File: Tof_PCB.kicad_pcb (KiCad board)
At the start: 4 copper layers, 115 x 65 mm, 275 parts, among them J1 Screw_Terminal_01x02, J2 Screw_Terminal_01x02, J3 Screw_Terminal_01x02, J4 Conn_02x03_Odd_Even, J5 Conn_01x04, J6 Conn_01x04, J7 Screw_Terminal_01x02, M1 mounting_holes_laser, M2 mounting_holes_laser, M3 mounting_holes_laser, M4 mounting_holes_laser, SW1 SW_Push, U1 ATmega328PB-MU, U10 NC7WZ00K8X, U11 UMCC_50Ohm, U12 UMCC_50Ohm, U13 NC7WZ00K8X, U14 NCP81074BDR2G, U15 LMH6559MF, U16 SiPM-MicroRB, U17 UMCC_50Ohm, U18 ts5a4596, U19 ts5a4596, U2 DAC128S085, U20 MAX40659, U21 LP5907MFX-3.3_NOPB, U22 UMCC_50Ohm, U23 TLV3501, U24 TLV3501, U25 HMC589AST89E, U26 NC7WZ00K8X, U27 UMCC_50Ohm, U28 UMCC_50Ohm, U29 UMCC_50Ohm, U3 LM4132BMF, U30 NC7WZ00K8X, U31 LM321, U32 UMCC_50Ohm, U33 UMCC_50Ohm, U34 NC7WZ16, U35 UMCC_50Ohm, U4 UMCC_50Ohm, U5 UMCC_50Ohm, U6 HMC589AST89E, U7 TLV3501, U8 UMCC_50Ohm, U9 NC7WZ00K8X, Y1 Crystal_GND24

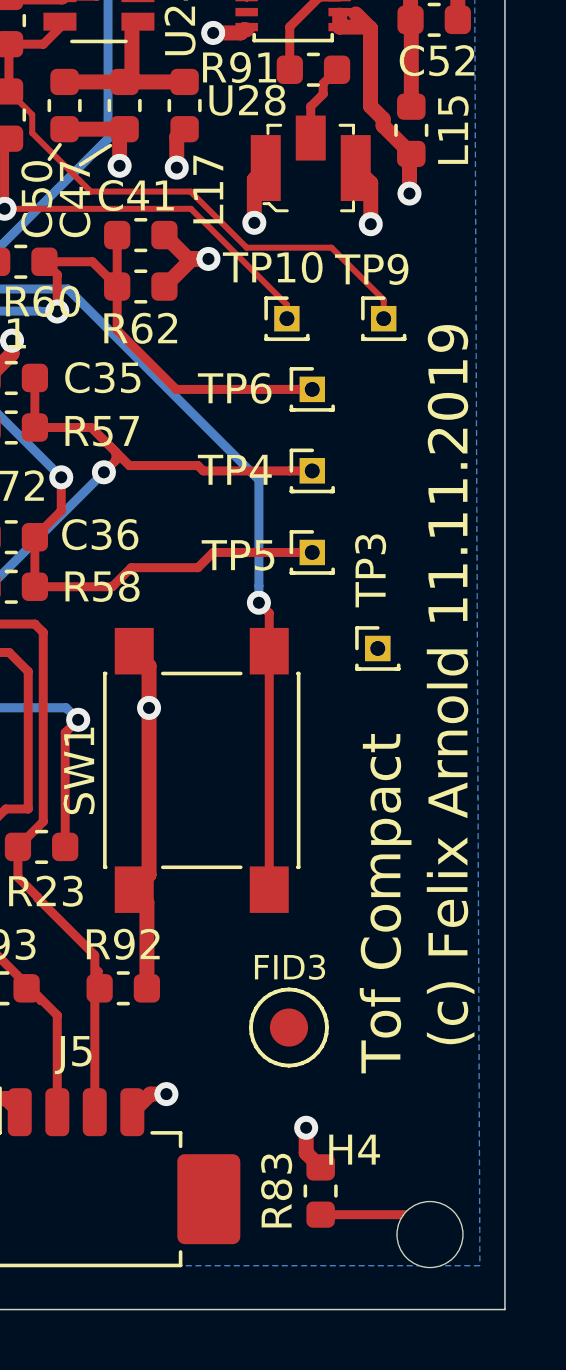
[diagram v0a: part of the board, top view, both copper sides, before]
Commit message: Version 1.0. As ordered at PCBWay on 13.11.2019
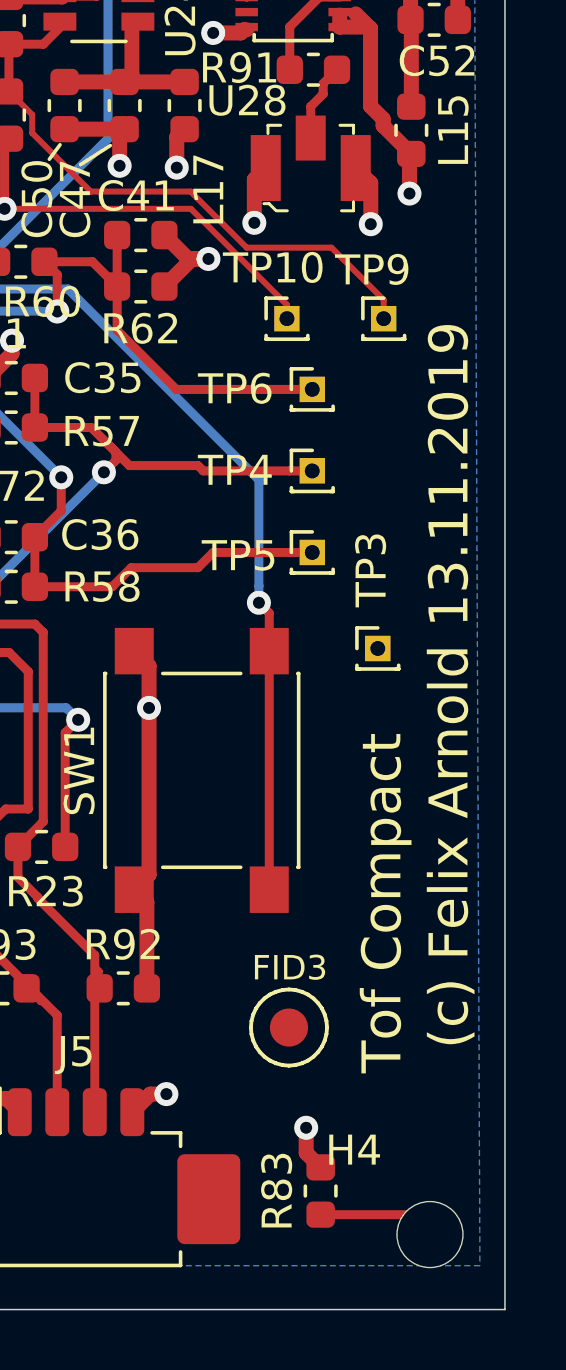
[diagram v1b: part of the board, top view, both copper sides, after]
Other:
- board text added: "(c) Felix Arnold 13.11.2019"
- board text removed: "(c) Felix Arnold 11.11.2019"
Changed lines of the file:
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@@
   (page A4)
   (layers
-    (0 F.Cu signal hide)
-    (1 In1.Cu mixed hide)
-    (2 In2.Cu mixed hide)
-    (31 B.Cu signal hide)
-    (32 B.Adhes user hide)
-    (33 F.Adhes user hide)
-    (34 B.Paste user hide)
-    (35 F.Paste user hide)
-    (36 B.SilkS user hide)
-    (37 F.SilkS user hide)
+    (0 F.Cu signal)
+    (1 In1.Cu mixed)
+    (2 In2.Cu mixed)
+    (31 B.Cu signal)
+    (32 B.Adhes user)
+    (33 F.Adhes user)
+    (34 B.Paste user)
+    (35 F.Paste user)
+    (36 B.SilkS user)
+    (37 F.SilkS user)
     (38 B.Mask user)
-    (39 F.Mask user hide)
-    (40 Dwgs.User user hide)
-    (41 Cmts.User user hide)
+    (39 F.Mask user)
+    (40 Dwgs.User user)
+    (41 Cmts.User user)
     (42 Eco1.User user)
     (43 Eco2.User user)
     (44 Edge.Cuts user)
-    (45 Margin user hide)
-    (46 B.CrtYd user hide)
+    (45 Margin user)
+    (46 B.CrtYd user)
     (47 F.CrtYd user)
-    (48 B.Fab user hide)
+    (48 B.Fab user)
     (49 F.Fab user)
   )
@@
       (outputformat 1)
       (mirror false)
-      (drillshape 1)
+      (drillshape 0)
       (scaleselection 1)
       (outputdirectory "outputs/"))
@@
   (gr_line (start 148.5265 60.3885) (end 151.511 60.3885) (layer F.SilkS) (width 0.12))
   (gr_line (start 146.812 54.61) (end 145.542 55.372) (layer F.SilkS) (width 0.12))
-  (gr_text "(c) Felix Arnold 11.11.2019" (at 168.148 94.1832 90) (layer F.SilkS)
+  (gr_text "(c) Felix Arnold 13.11.2019" (at 168.148 94.1832 90) (layer F.SilkS)
     (effects (font (size 1.3 1.3) (thickness 0.25)))
   )
